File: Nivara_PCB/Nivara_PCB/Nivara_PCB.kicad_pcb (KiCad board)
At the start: 4 copper layers, 98.8 x 81.2 mm, 167 parts, among them CN1 ANALOG_IN, CN2 RELAY, J1 AUXILIAR, K1 SRA-24VDC-CL, K2 SRA-24VDC-CL, P1 NPN_IN, P2 PNP_IN, P3 D_IN, P4 RUN/STOP, P5 NPN_OUT, P6 PNP_OUT, P7 RS485, P8 ANALOG_OUT., Q1 IRLML0040, Q2 AO3407A, Q3 IRLML0040, Q4 AO3407A, Q5 IRLML6402TRPBF-JSM, SW1 SKRPACE010, SW2 SKRPACE010, U1 2.54-2*2, U10 GP8201S-TC50-EW, U11 LK1802, U12 LTV-357T, U13 LTV-357T, U14 LTV-357T, U15 LTV-357T, U16 LTV-357T, U17 LTV-357T, U18 LTV-357T, U19 GP8303-TC50-EW, U2 FUENTE IN, U20 FUENTE EX, U3 ESP32-S3-WROOM-1, U4 AP63200WU, U5 RSM3485ECHT_C2992406, U6 LTV-357T, U7 LTV-357T, U8 LTV-357T, U9 LTV-357T

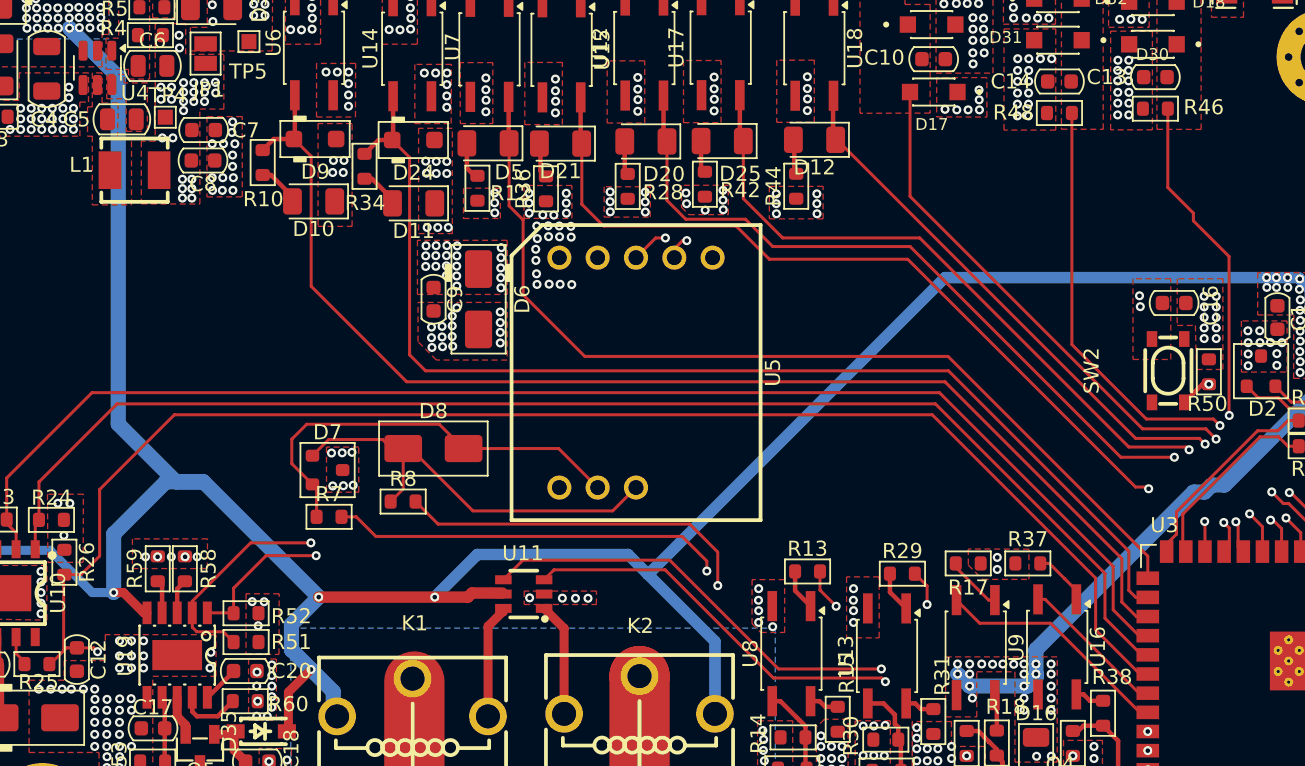
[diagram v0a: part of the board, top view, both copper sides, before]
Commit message: PCB listo para revisión.
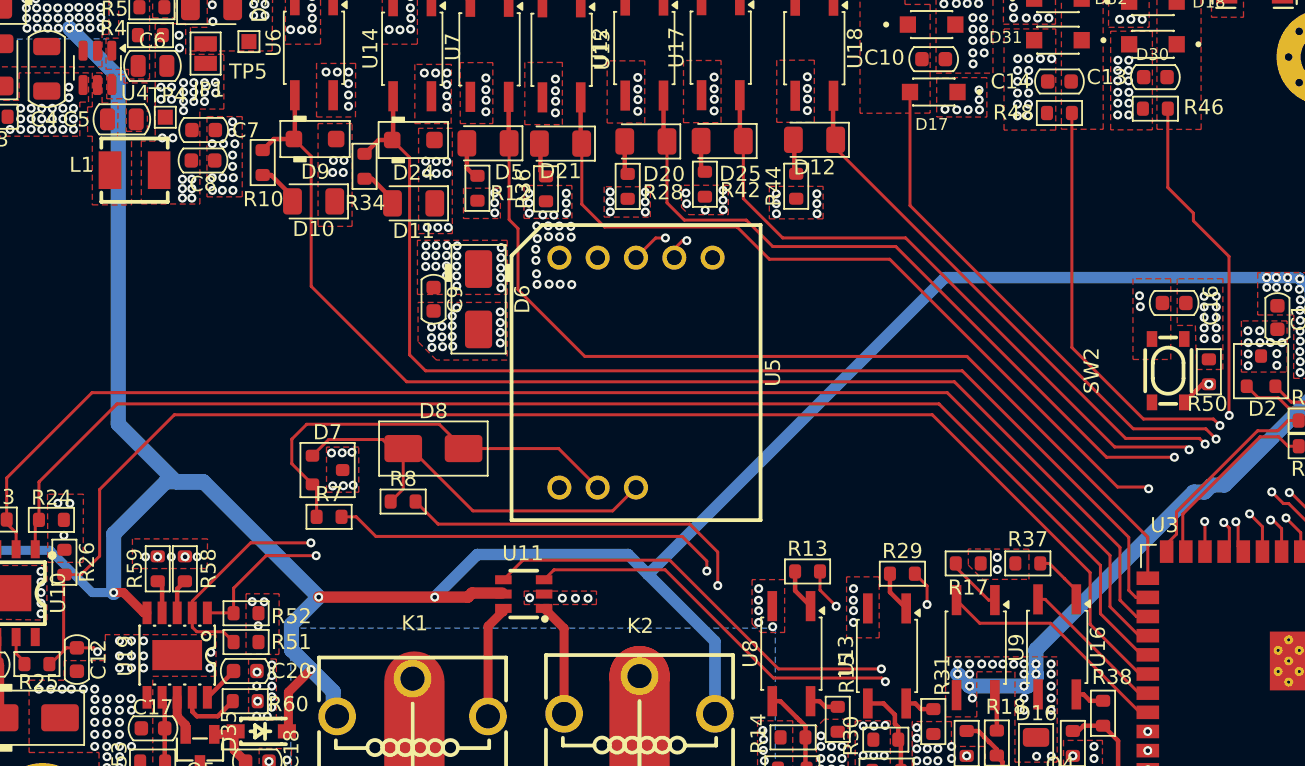
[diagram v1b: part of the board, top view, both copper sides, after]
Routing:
- net /NIVARA_BOARD/PNP_IN_1/PNP_OUT: track 63.4 -> 64.1 mm
- net /NIVARA_BOARD/NPN_IN_2/NPN_OUT: track 77.1 -> 77.7 mm
